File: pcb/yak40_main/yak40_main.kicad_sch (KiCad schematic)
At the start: 139 parts, among them J1 Conn_01x04, J2 Conn_01x03_Pin, SW1 SW_Push, SW10 SW_Push, SW11 SW_Push, SW12 SW_Push, SW13 SW_Push, SW14 SW_Push, SW15 SW_Push, SW16 SW_Push, SW17 SW_Push, SW18 SW_Push, SW19 SW_Push, SW2 SW_Push, SW20 SW_Push, SW21 SW_Push, SW22 SW_Push, SW23 SW_Push, SW24 SW_Push, SW25 SW_Push, SW26 SW_Push, SW27 SW_Push, SW28 SW_Push, SW29 SW_Push, SW3 SW_Push, SW30 SW_Push, SW31 SW_Push, SW32 SW_Push, SW33 SW_Push, SW34 SW_Push, SW35 SW_Push, SW36 SW_Push, SW37 SW_Push, SW38 SW_Push, SW39 SW_Push, SW4 SW_Push, SW40 SW_Push, SW41 SW_Push, SW42 SW_Push, SW43 SW_Push, SW44 SW_Push, SW45 SW_Push, SW46 SW_Push, SW47 SW_Push, SW48 SW_Push, SW49 SW_Push, SW5 SW_Push, SW50 SW_Push, SW51 SW_Push, SW52 SW_Push, SW53 SW_Push, SW54 SW_Push, SW55 SW_Push, SW6 SW_Push, SW7 SW_Push, SW8 SW_Push, SW9 SW_Push, U1 NCP1117-3.3_SOT223, U2 RP2040, U3 W25Q128JVS, Y1 Crystal

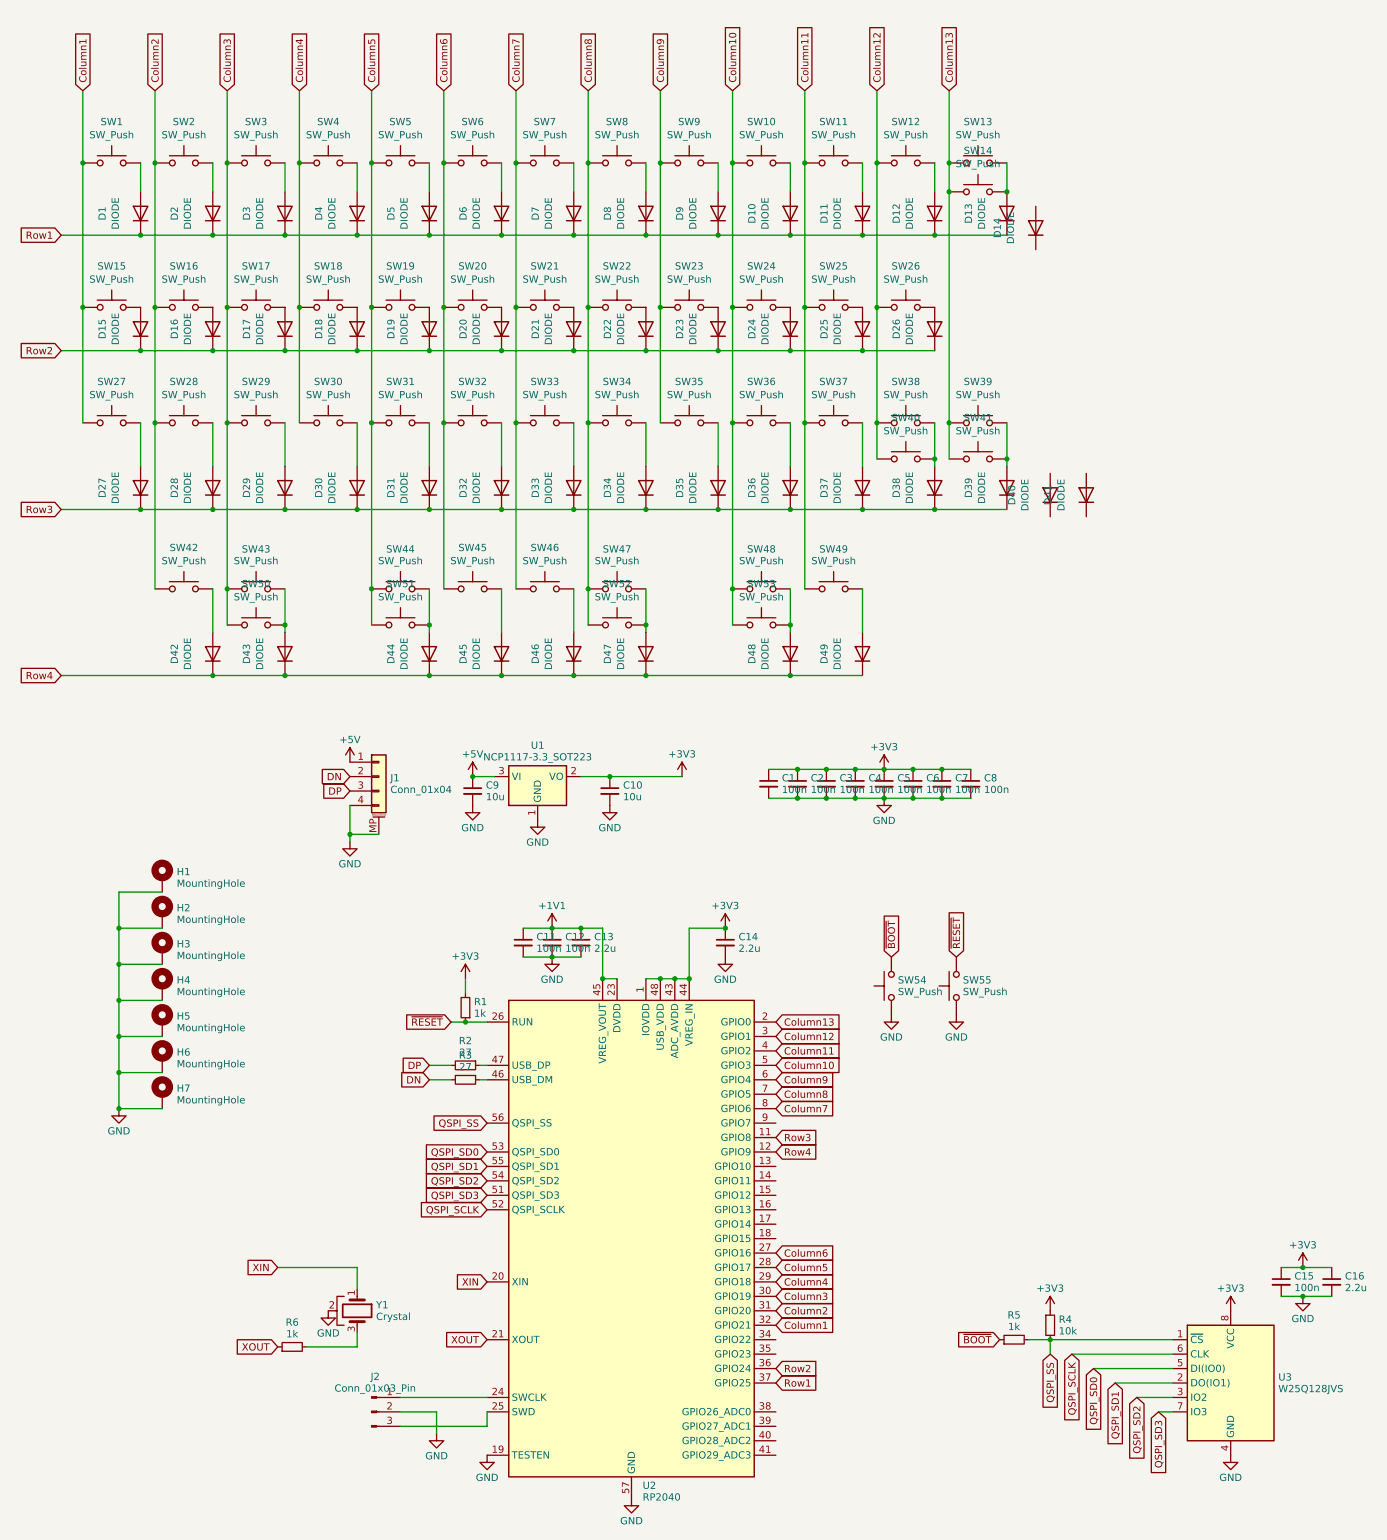
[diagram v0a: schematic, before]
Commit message: Update pcb
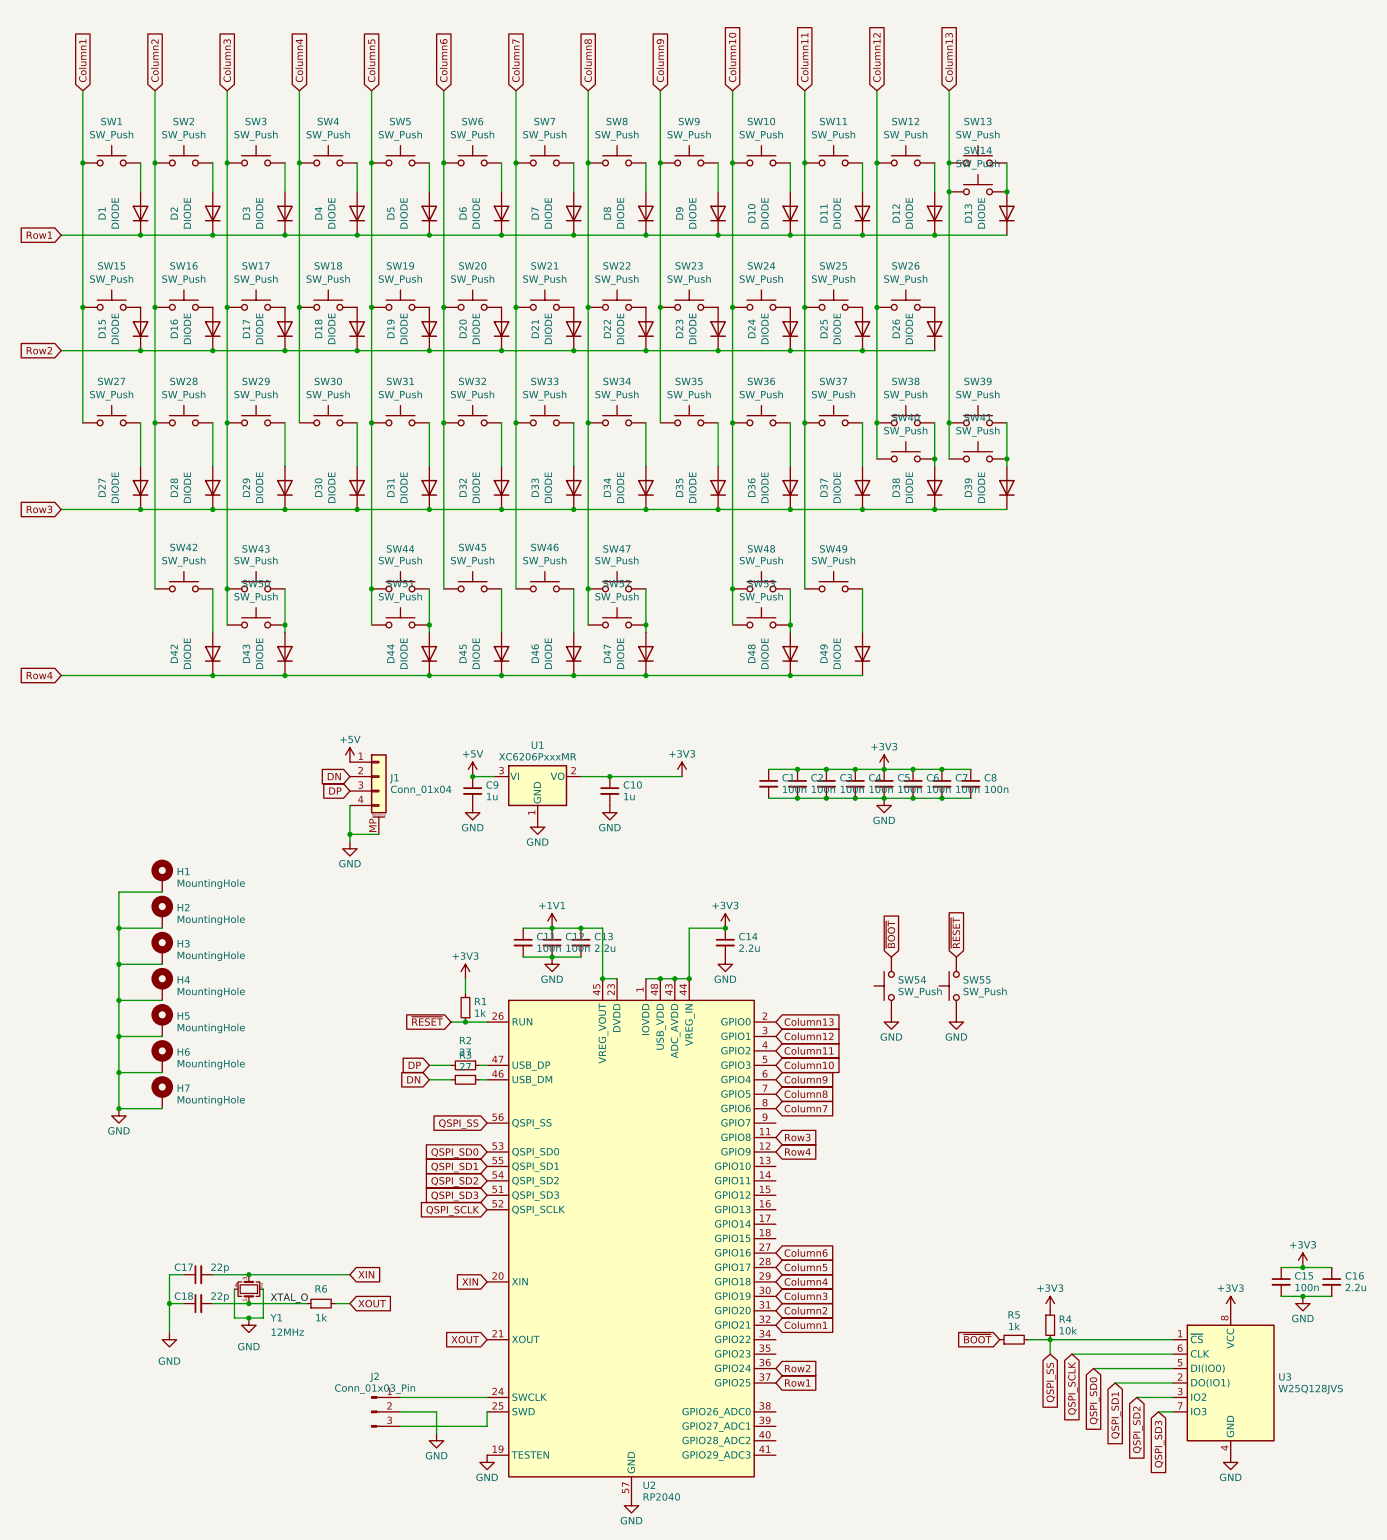
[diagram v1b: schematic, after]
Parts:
- removed D14, D40, D41: DIODE, Diode_SMD:D_1206_3216Metric_Pad1.42x1.75mm_HandSolder, symbol Diode:1N4148W
- removed U1: NCP1117-3.3_SOT223, Package_TO_SOT_SMD:SOT-223-3_TabPin2, symbol Regulator_Linear:NCP1117-3.3_SOT223
- removed Y1: Crystal, Crystal:Resonator_SMD_Murata_CSTxExxV-3Pin_3.0x1.1mm_HandSoldering, symbol Device:Crystal_GND2
- added C17, C18: 22p, Capacitor_SMD:C_0402_1005Metric, symbol Device:C_Small
- added U1: XC6206PxxxMR, Package_TO_SOT_SMD:SOT-23-3, symbol Regulator_Linear:XC6206PxxxMR
- added Y1: 12MHz, Crystal:Crystal_SMD_3225-4Pin_3.2x2.5mm, symbol Device:Crystal_GND24_Small
- C10, C9: value 10u -> 1u
- D1, D10, D11, D12, D13, D15, D16, D17, D18, D19, D2, D20, D21, D22, D23, D24, D25, D26, D27, D28, D29, D3, D30, D31, D32, D33, D34, D35, D36, D37, D38, D39, D4, D42, D43, D44, D45, D46, D47, D48, D49, D5, D6, D7, D8, D9: footprint Diode_SMD:D_1206_3216Metric_Pad1.42x1.75mm_HandSolder -> Diode_SMD:D_SOD-123
- R6: LCSC (none) -> C11702
- SW54, SW55: footprint Button_Switch_SMD:SW_Push_1P1T_NO_Vertical_Wuerth_434133025816 -> Button_Switch_SMD:SW_Push_1P1T_XKB_TS-1187A
- U3: footprint Package_SON:WSON-8-1EP_6x5mm_P1.27mm_EP3.4x4.3mm -> Package_SO:SOIC-8_5.23x5.23mm_P1.27mm
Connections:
- net +3V3: now also U1.2 (VO)
- net +5V: now also U1.3 (VI)
- net GND: now also C17.1, C18.1, U1.1 (GND), Y1.2, Y1.4
- net XIN: now also C17.2, Y1.3
- net XOUT: now also R6.2; no longer R6.1
- new net XTAL_O: C18.2, R6.1, Y1.1
